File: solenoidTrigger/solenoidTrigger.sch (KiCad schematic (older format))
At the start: 40 parts, among them J3 CONN_01X03, J4 UF_2_RA, J5 micromatch, J6 CONN_01X03, J7 CONN_01X03, J8 CONN_02X03, Q1 NMOS_CDS16, Q2 NMOS_CDS16, Q3 NMOS_CDS16, Q4 NMOS_CDS16, Q5 NMOS_CDS16, Q6 NMOS_CDS16, U1 L78M05CDT-TR, U2 ATmega328P-AU, Y2 Crystal_SMD

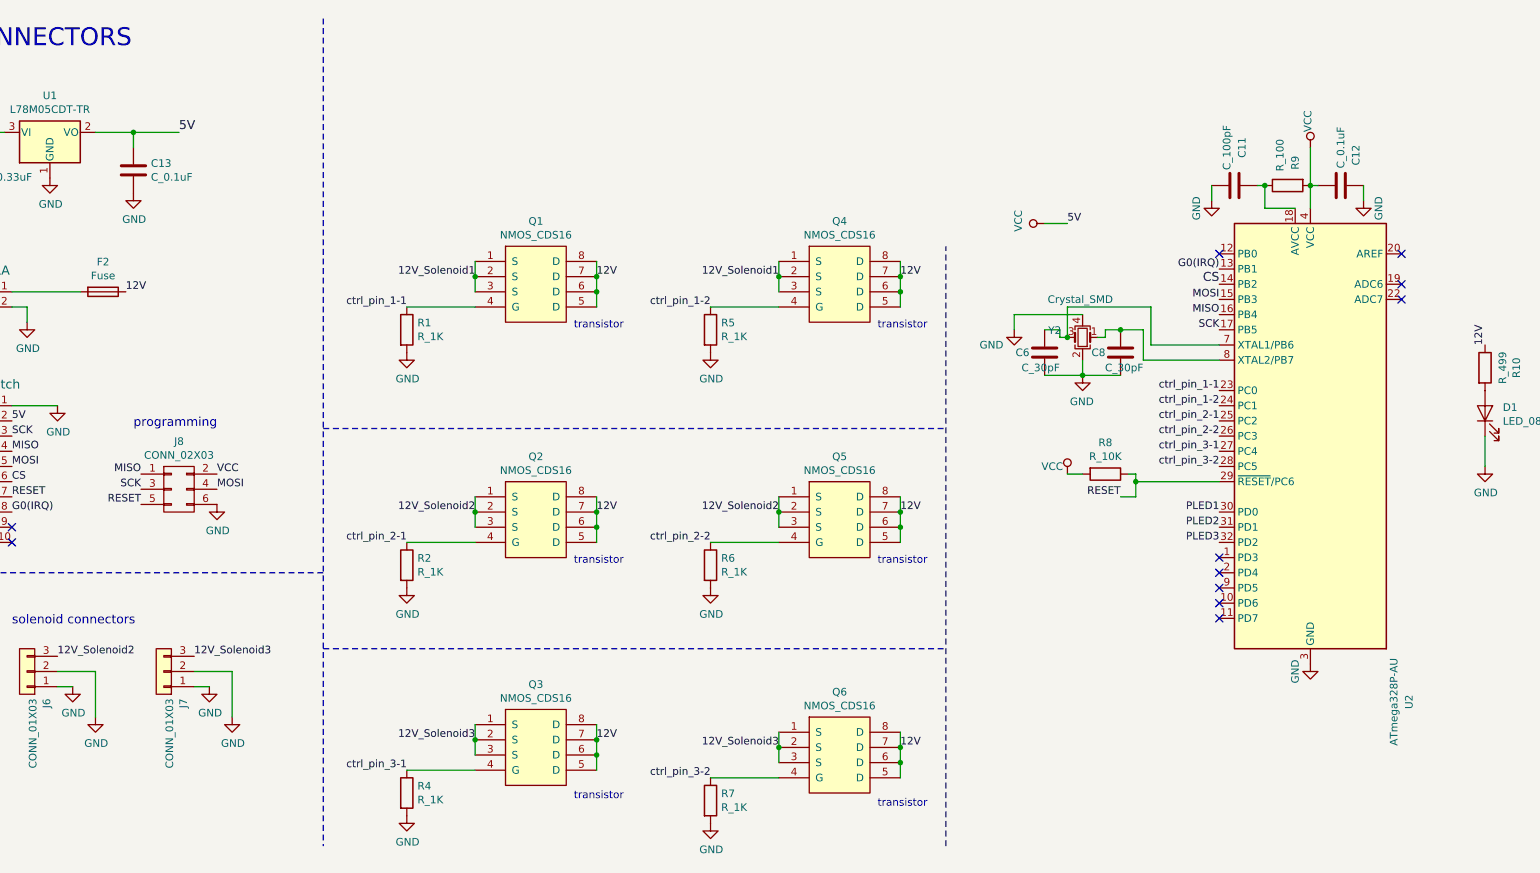
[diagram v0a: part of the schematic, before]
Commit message: Updated with no errors
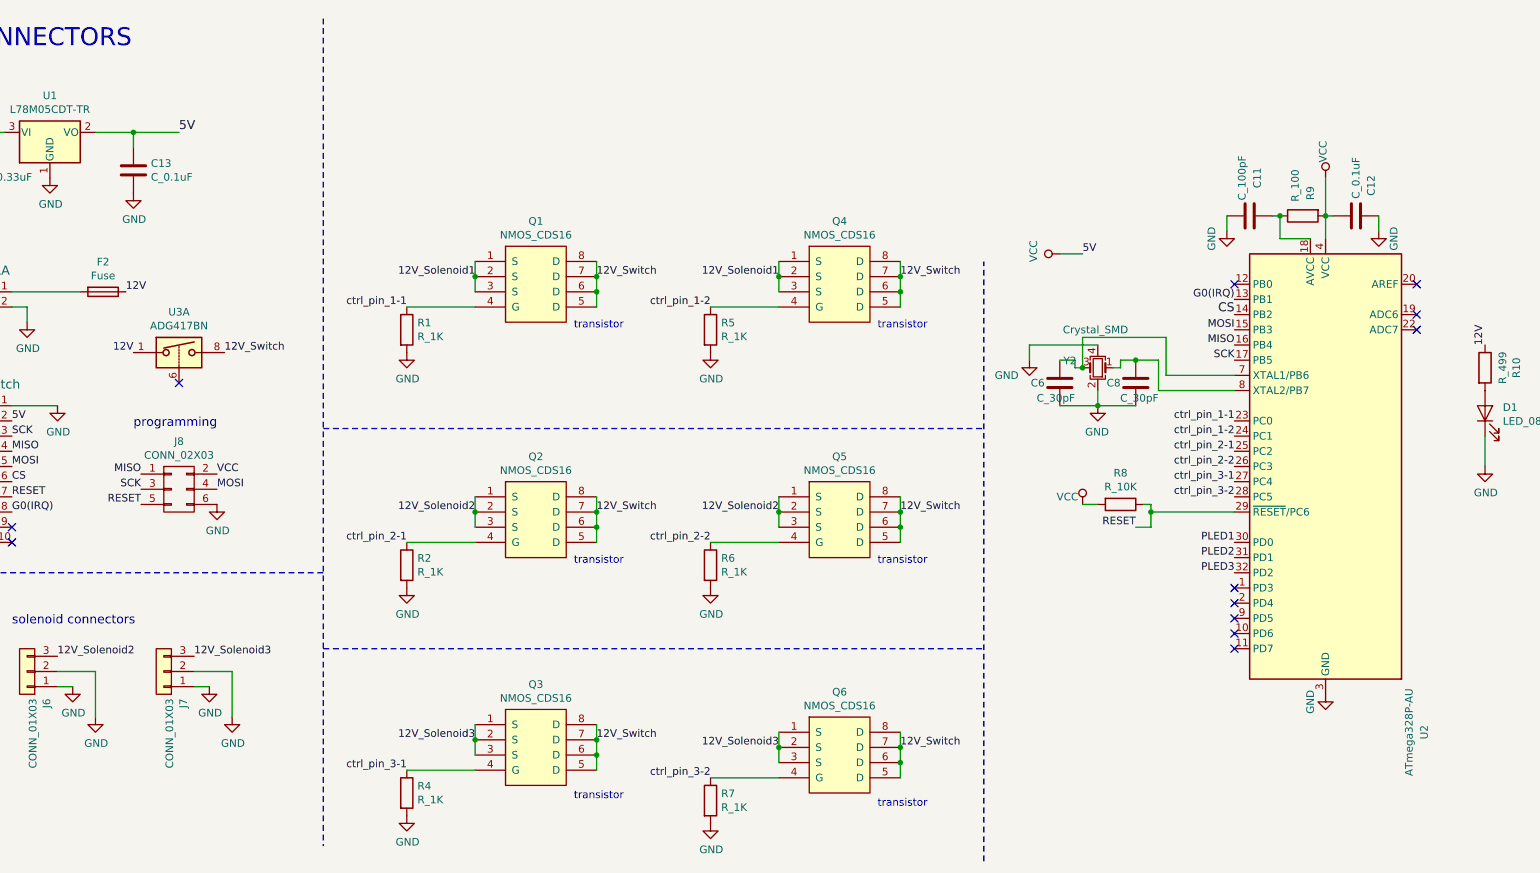
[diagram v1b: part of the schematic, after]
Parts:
- added U3: ADG417BN, Package_DIP:DIP-8_W7.62mm, symbol Analog_Switch:ADG417BN
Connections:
- net 12V: now also U3.1; no longer Q1.5 (D), Q1.6 (D), Q1.7 (D), Q1.8 (D), Q2.5 (D), Q2.6 (D), Q2.7 (D), Q2.8 (D), Q3.5 (D), Q3.6 (D), Q3.7 (D), Q3.8 (D), Q4.5 (D), Q4.6 (D), Q4.7 (D), Q4.8 (D), Q5.5 (D), Q5.6 (D), Q5.7 (D), Q5.8 (D), Q6.5 (D), Q6.6 (D), Q6.7 (D), Q6.8 (D)
- new net 12V_Switch: Q1.5 (D), Q1.6 (D), Q1.7 (D), Q1.8 (D), Q2.5 (D), Q2.6 (D), Q2.7 (D), Q2.8 (D), Q3.5 (D), Q3.6 (D), Q3.7 (D), Q3.8 (D), Q4.5 (D), Q4.6 (D), Q4.7 (D), Q4.8 (D), Q5.5 (D), Q5.6 (D), Q5.7 (D), Q5.8 (D), Q6.5 (D), Q6.6 (D), Q6.7 (D), Q6.8 (D), U3.8
- no-connect marks 11 -> 12
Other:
- moved on the sheet: C11, C12, C6, C8, R8, R9, U2, Y2
